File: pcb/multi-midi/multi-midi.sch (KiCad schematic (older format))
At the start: 60 parts, among them J1 USB_B_Mini, J10 DIN-5_180degree, J11 DIN-5_180degree, J12 DIN-5_180degree, J13 DIN-5_180degree, J14 DIN-5_180degree, J15 AudioJack3, J16 AudioJack3, J17 AudioJack3, J18 AudioJack3, J19 AudioJack3, J2 DIN-5_180degree, J20 AudioJack3, J21 AudioJack3, J22 AudioJack3, J23 AudioJack3, J24 AudioJack3, J25 AudioJack3, J26 AudioJack3, J3 DIN-5_180degree, J4 DIN-5_180degree, J5 DIN-5_180degree, J6 DIN-5_180degree, J7 DIN-5_180degree, J8 DIN-5_180degree, J9 DIN-5_180degree, U1 6N137, U2 4050, U3 4050

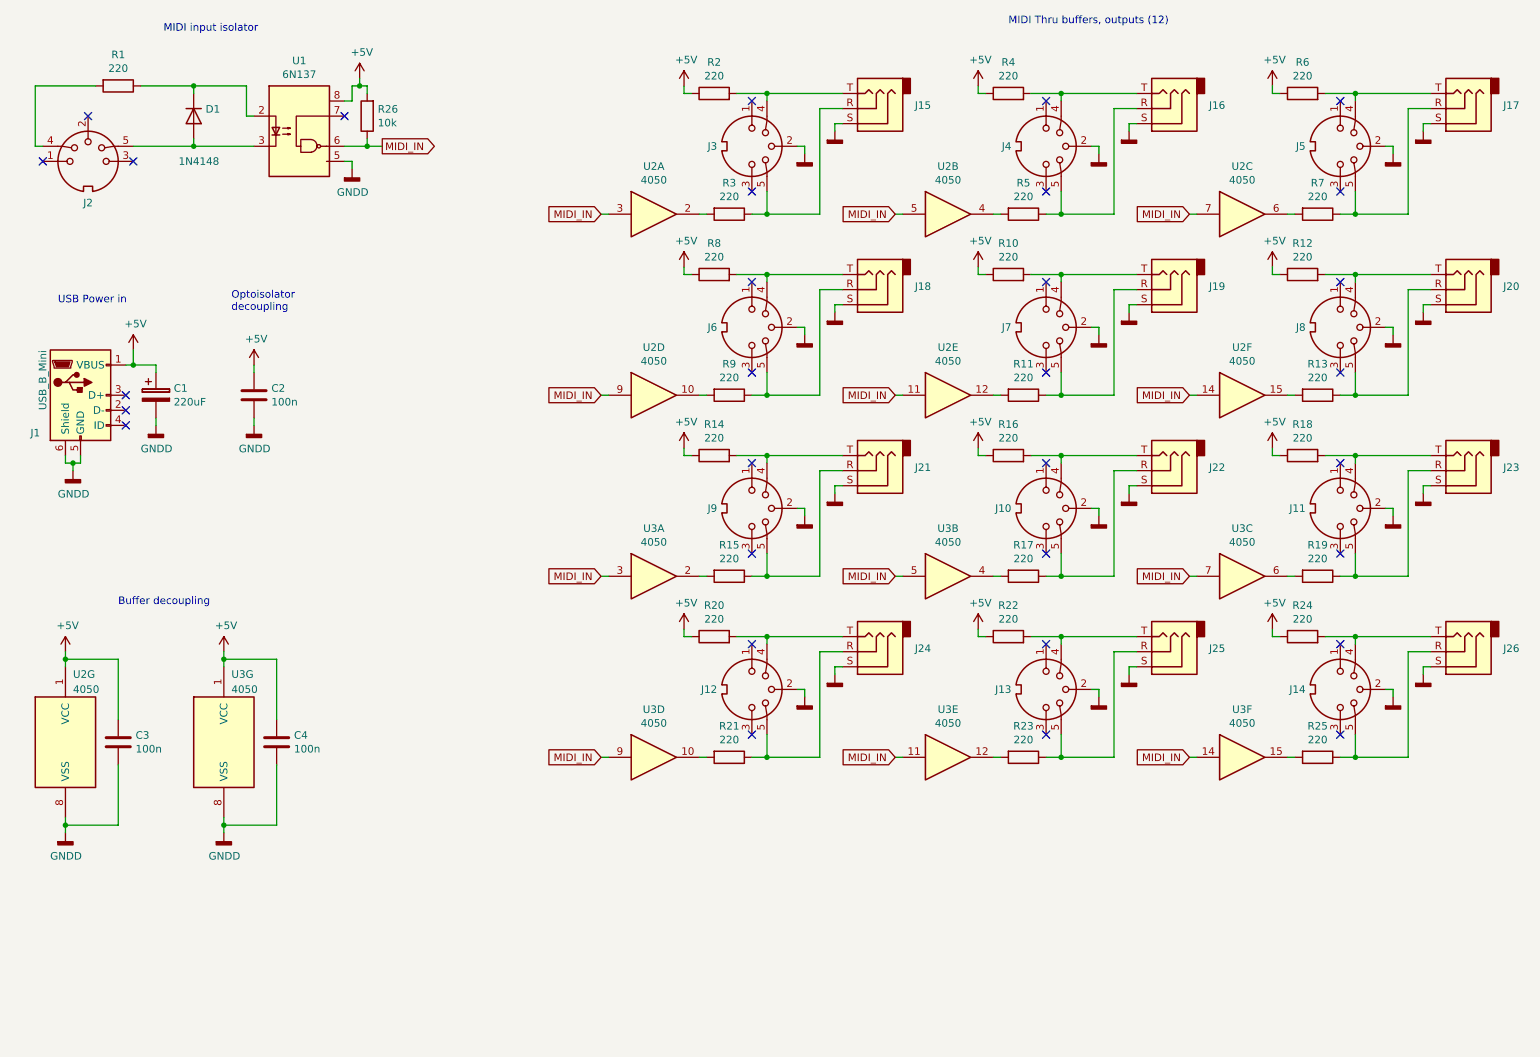
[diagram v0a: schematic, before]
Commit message: Actually do this. Redrew schematic, design PCB
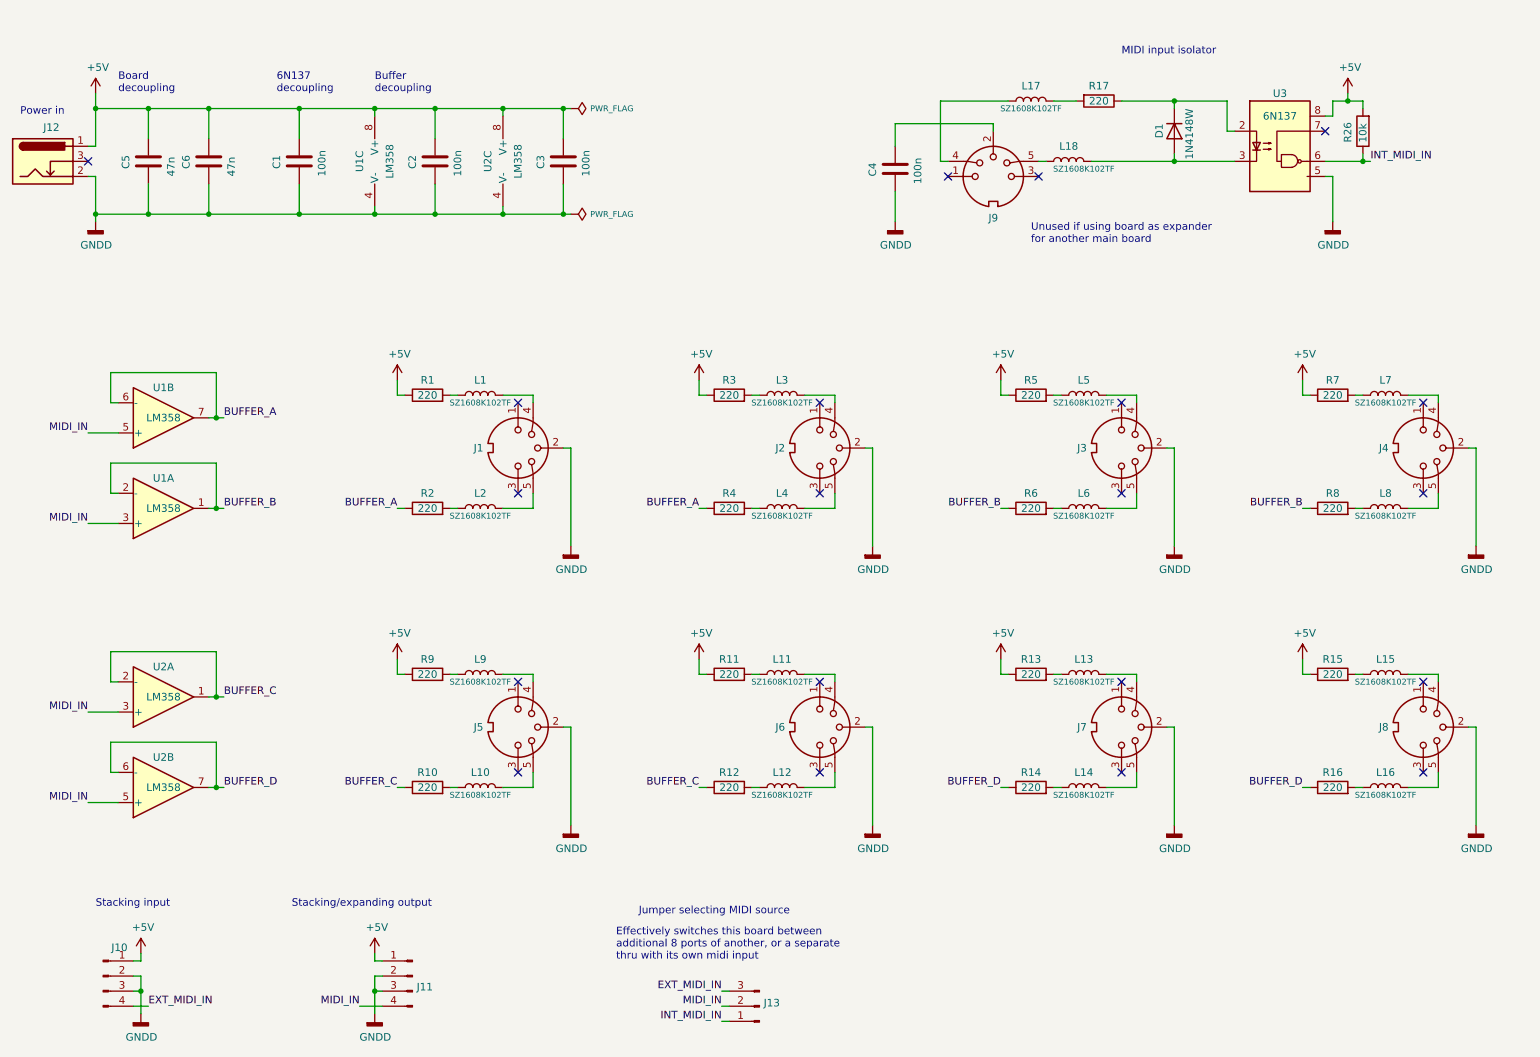
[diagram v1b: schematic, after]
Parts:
- removed C1: 220uF, symbol Device:CP
- removed J1: USB_B_Mini, symbol Connector:USB_B_Mini
- removed J10, J11, J12, J13, J14, J9: DIN-5_180degree, symbol Connector:DIN-5_180degree
- removed J15, J16, J17, J18, J19, J20, J21, J22, J23, J24, J25, J26: AudioJack3, symbol Connector:AudioJack3
- removed R17, R18, R19, R20, R21, R22, R23, R24, R25: 220, symbol Device:R
- removed U2, U3: 4050, symbol 4xxx:4050
- added C2: 100n, Capacitor_SMD:C_0603_1608Metric, symbol Device:C
- added C5, C6: 47n, Capacitor_SMD:C_1206_3216Metric, symbol Device:C
- added J1, J2: DIN-5_180degree, multi-midi:DIN-5, symbol Connector:DIN-5_180degree
- added J10, J11: Conn_01x04_Male, Connector_JST:JST_EH_S4B-EH_1x04_P2.50mm_Horizontal, symbol Connector:Conn_01x04_Male
- added J12: Barrel_Jack_Switch, Connector_BarrelJack:BarrelJack_Wuerth_6941xx301002, symbol Connector:Barrel_Jack_Switch
- added J13: Conn_01x03_Male, Connector_PinHeader_2.54mm:PinHeader_1x03_P2.54mm_Vertical, symbol Connector:Conn_01x03_Male
- added L1, L10, L11, L12, L13, L14, L15, L16, L17, L2, L3, L4, L5, L6, L7, L8, L9: SZ1608K102TF, Inductor_SMD:L_0603_1608Metric, symbol Device:L
- added L18: SZ1608K102TF, Resistor_SMD:R_0603_1608Metric, symbol Device:L
- added R1: 220, Resistor_SMD:R_0603_1608Metric, symbol Device:R
- added U1, U2: LM358, Package_SO:SOIC-8_3.9x4.9mm_P1.27mm, symbol Amplifier_Operational:LM358
- C1: renamed from C2; footprint (none) -> Capacitor_SMD:C_0603_1608Metric; LCSC (none) -> C14663
- C3, C4: footprint (none) -> Capacitor_SMD:C_0603_1608Metric; LCSC (none) -> C14663
- D1: value 1N4148 -> 1N4148W; footprint Diode_THT:D_DO-35_SOD27_P7.62mm_Horizontal -> Diode_SMD:D_SOD-123; LCSC (none) -> C81598
- J3, J4, J5, J6, J7, J8: footprint (none) -> multi-midi:DIN-5
- J9: renamed from J2; footprint (none) -> multi-midi:DIN-5
- R10, R11, R12, R13, R14, R15, R16, R2, R3, R4, R5, R6, R7, R8, R9: footprint (none) -> Resistor_SMD:R_0603_1608Metric; LCSC (none) -> C22962
- R17: renamed from R1; footprint (none) -> Resistor_SMD:R_0603_1608Metric; LCSC (none) -> C22962
- R26: footprint (none) -> Resistor_SMD:R_0603_1608Metric; LCSC (none) -> C25804
- U3: renamed from U1; footprint (none) -> Package_SO:SSO-8_6.7x9.8mm_P2.54mm_Clearance8mm; LCSC (none) -> C110020
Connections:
- net +5V: now also R11.1, R13.1, R15.1, R3.1, R5.1, R7.1, R9.1, C2.1, C5.1, C6.1, J10.1 (Pin_1), J11.1 (Pin_1), J12.1, R1.1, U1.8 (V+), U2.8 (V+); no longer C4.1, R10.1, R12.1, R14.1, R16.1, R2.1, R4.1, R6.1, R8.1
- net GNDD: now also C2.2, C5.2, C6.2, J1.2, J10.2 (Pin_2), J10.3 (Pin_3), J11.2 (Pin_2), J11.3 (Pin_3), J12.2, J2.2, U1.4 (V-), U2.4 (V-)
- net MIDI_IN: now also J11.4 (Pin_4), J13.2 (Pin_2), U1.3 (+), U1.5 (+), U2.3 (+), U2.5 (+); no longer R26.1, U3.6 (VO2)
- net at D1.2 (A), U3.3 (C2): now also L18.2; no longer J9.5
- net at R2.2: now also L2.1; no longer J3.4
- net at J3.5: now also L6.2; no longer R3.1
- net at J9.2: now also C4.1
- net at J9.4: now also L17.1; no longer R17.2
- net at R3.2: now also L3.1
- net at R4.2: now also L4.1; no longer J4.4
- net at J4.5: now also L8.2; no longer R5.1
- net at R5.2: now also L5.1
- net at R6.2: now also L6.1; no longer J5.4
- net at J5.5: now also L10.2; no longer R7.1
- net at R7.2: now also L7.1
- net at R8.2: now also L8.1; no longer J6.4
- net at J6.5: now also L12.2; no longer R9.1
- net at R9.2: now also L9.1
- net at R10.2: now also L10.1; no longer J7.4
- net at J7.5: now also L14.2; no longer R11.1
- net at R11.2: now also L11.1
- net at R12.2: now also L12.1; no longer J8.4
- net at J8.5: now also L16.2; no longer R13.1
- net at R13.2: now also L13.1
- net at R14.2: now also L14.1
- net at R15.2: now also L15.1
- net at R16.2: now also L16.1
- new net: J9.5, L18.1
- new net: L17.2, R17.2
- new net: J1.4, L1.2
- new net: J1.5, L2.2
- new net: L1.1, R1.2
- new net: J2.4, L3.2
- new net: J2.5, L4.2
- new net: J3.4, L5.2
- new net: J4.4, L7.2
- new net: J5.4, L9.2
- new net: J6.4, L11.2
- new net: J7.4, L13.2
- new net: J8.4, L15.2
- new net BUFFER_A: R2.1, R4.1, U1.6 (-), U1.7
- new net BUFFER_B: R6.1, R8.1, U1.1, U1.2 (-)
- new net BUFFER_C: R10.1, R12.1, U2.1, U2.2 (-)
- new net BUFFER_D: R14.1, R16.1, U2.6 (-), U2.7
- new net EXT_MIDI_IN: J10.4 (Pin_4), J13.3 (Pin_3)
- new net INT_MIDI_IN: J13.1 (Pin_1), R26.1, U3.6 (VO2)
- no-connect marks 31 -> 20
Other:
- note added: "6N137\ndecoupling\n"
- note added: "Board\ndecoupling"
- note added: "Buffer\ndecoupling"
- note added: "Effectively switches this board between\nadditional 8 ports of another, or a separate\nthru with its own midi input"
- note added: "Jumper selecting MIDI source"
- note added: "Power in"
- note added: "Stacking input"
- note added: "Stacking/expanding output"
- note added: "Unused if using board as expander \nfor another main board"
- note removed: "Buffer decoupling"
- note removed: "MIDI Thru buffers, outputs (12)"
- note removed: "Optoisolator\ndecoupling\n"
- note removed: "USB Power in"
- moved on the sheet: C1, D1, J9, R17, R26, U3
